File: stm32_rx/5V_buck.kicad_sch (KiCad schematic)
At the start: 13 parts

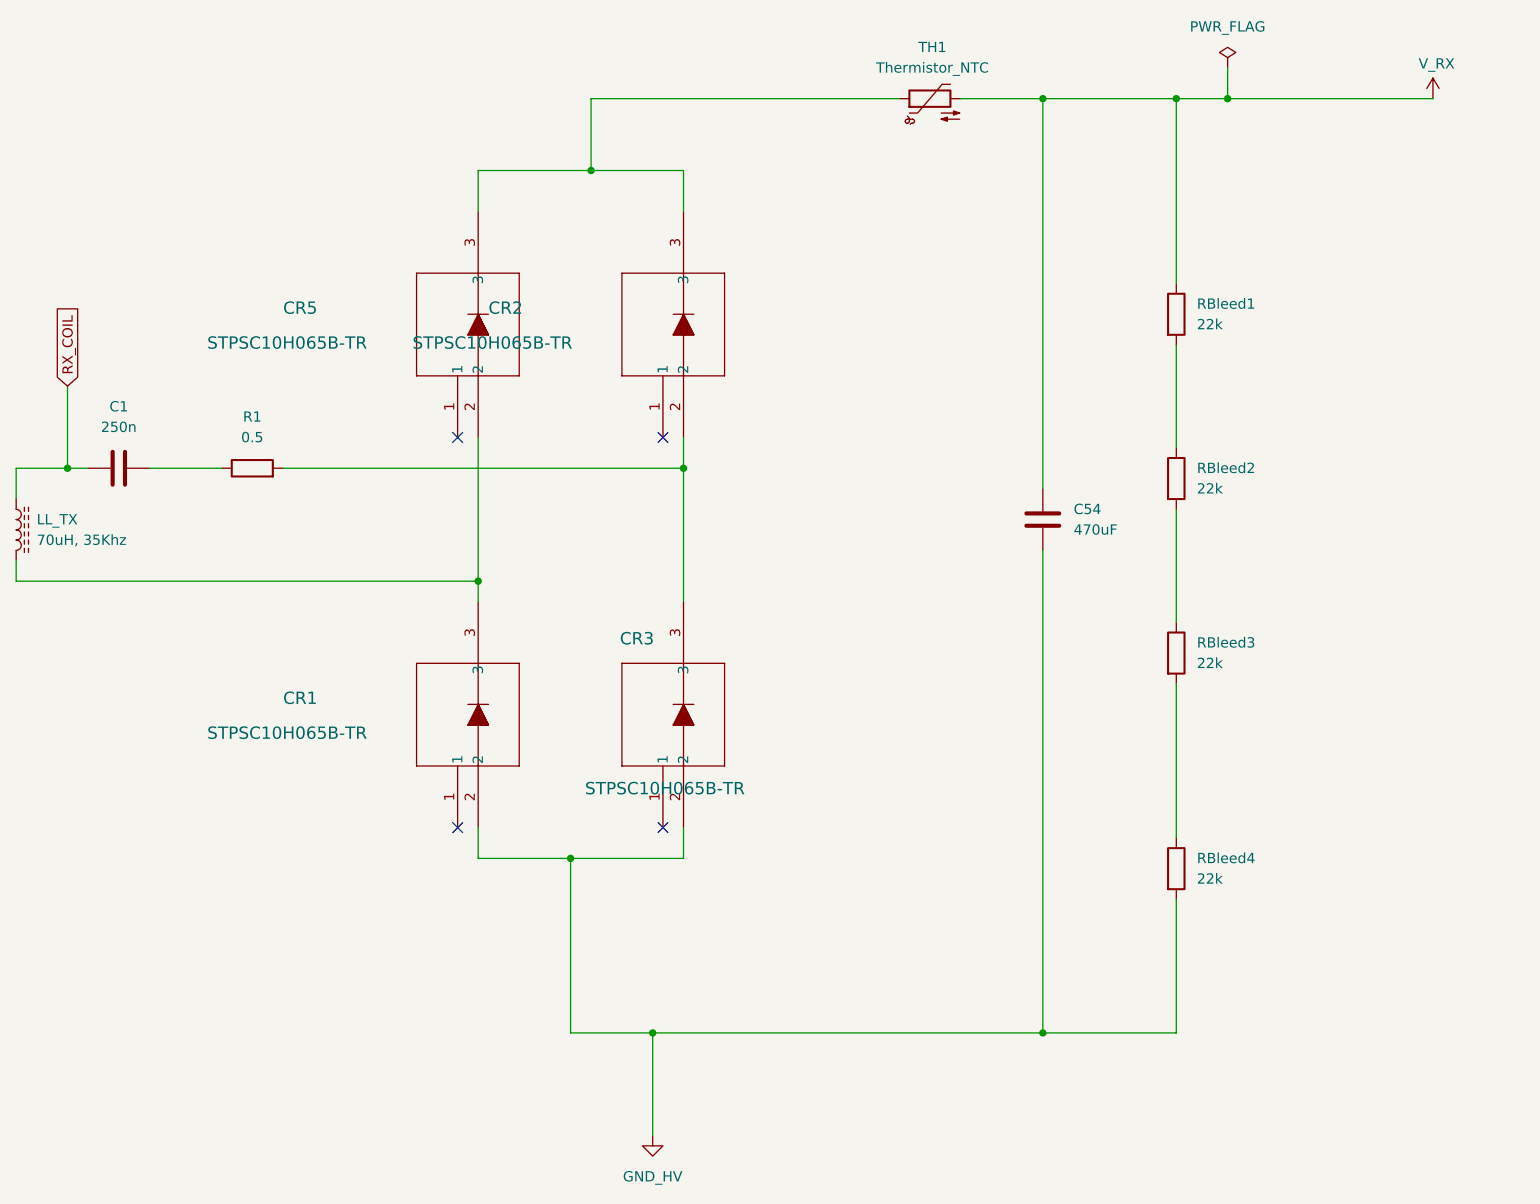
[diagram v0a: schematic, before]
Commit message: I can't find the right module
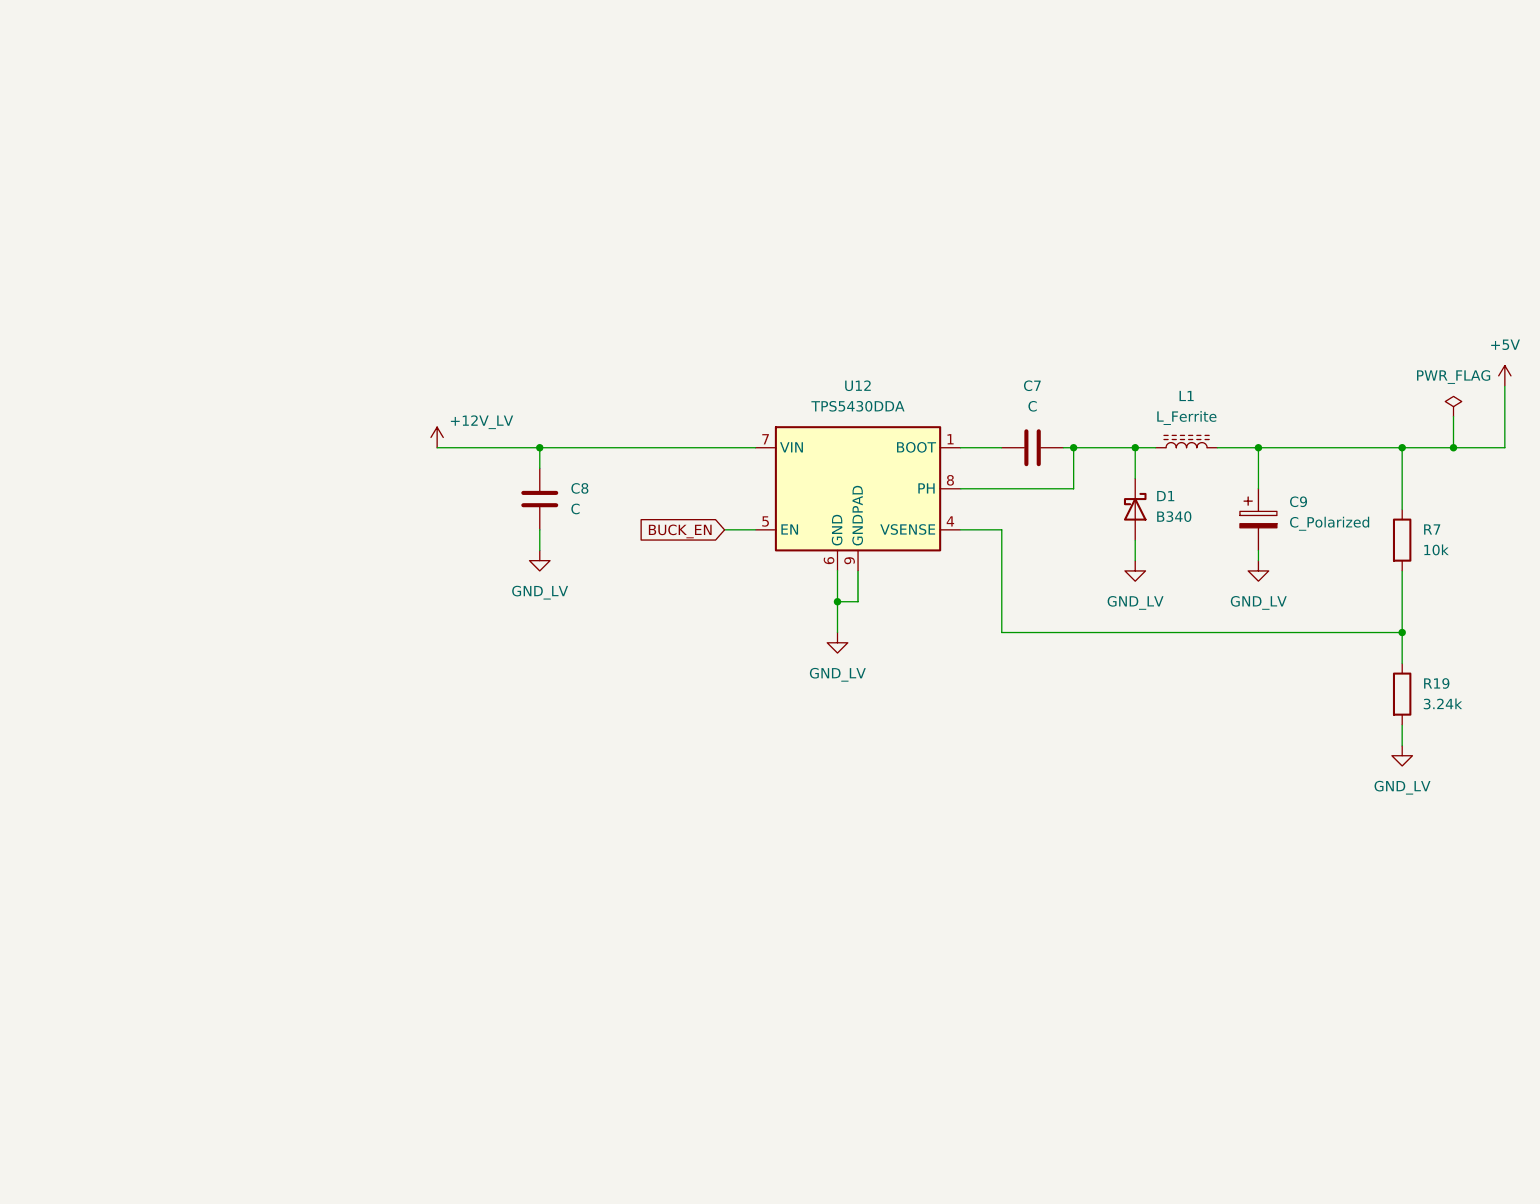
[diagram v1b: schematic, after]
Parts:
- removed C1: 250n, symbol Device:C
- removed C54: 470uF, symbol Device:C
- removed CR1, CR2, CR3, CR5: STPSC10H065B-TR, WPT_TX:DPAK_STPS_STM, symbol 2026-07-24_14-19-21:STPSC10H065B-TR
- removed LL_TX: 70uH, 35Khz, symbol Device:L_Ferrite
- removed R1: 0.5, symbol Device:R
- removed RBleed1, RBleed2, RBleed3, RBleed4: 22k, symbol Device:R
- removed TH1: Thermistor_NTC, symbol Device:Thermistor_NTC
- added C7: C, Capacitor_SMD:C_0402_1005Metric, symbol Device:C
- added C8: C, symbol Device:C
- added C9: C_Polarized, symbol Device:C_Polarized
- added D1: B340, Diode_SMD:D_SMC, symbol Diode:B340
- added L1: L_Ferrite, symbol Device:L_Ferrite
- added R19: 3.24k, symbol Device:R
- added R7: 10k, symbol Device:R
- added U12: TPS5430DDA, Package_SO:TI_SO-PowerPAD-8_ThermalVias, symbol Regulator_Switching:TPS5430DDA
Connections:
- new net: R19.1, R7.2, U12.4 (VSENSE)
- new net: C7.2, D1.1 (K), L1.1, U12.8 (PH)
- new net: C7.1, U12.1 (BOOT)
- new net +12V_LV: C8.1, U12.7 (VIN)
- new net +5V: C9.1, L1.2, R7.1
- new net BUCK_EN: U12.5 (EN)
- new net GND_LV: C8.2, C9.2, D1.2 (A), R19.2, U12.6 (GND), U12.9 (GNDPAD)
- no-connect marks 4 -> 0
